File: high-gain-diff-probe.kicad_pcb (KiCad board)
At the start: 2 copper layers, 110 x 80 mm, 94 parts, among them J1 30V DC IN, J2 BNC, J4 BNC, J5 BNC, K1 FTR-B3SA012Z, K2 FTR-B3SA012Z, Q1 2N3906, SW1 MB04L1NCGD, SW2 MB05L1NCGD, SW3 SPDT, SW4 MB04L1NCGD, SW6 SPDT, U1 AD8428BRZ, U2 OP1177AR, U3 BUF634A, U6 LM393, U7 AD8671, U8 BUF634A

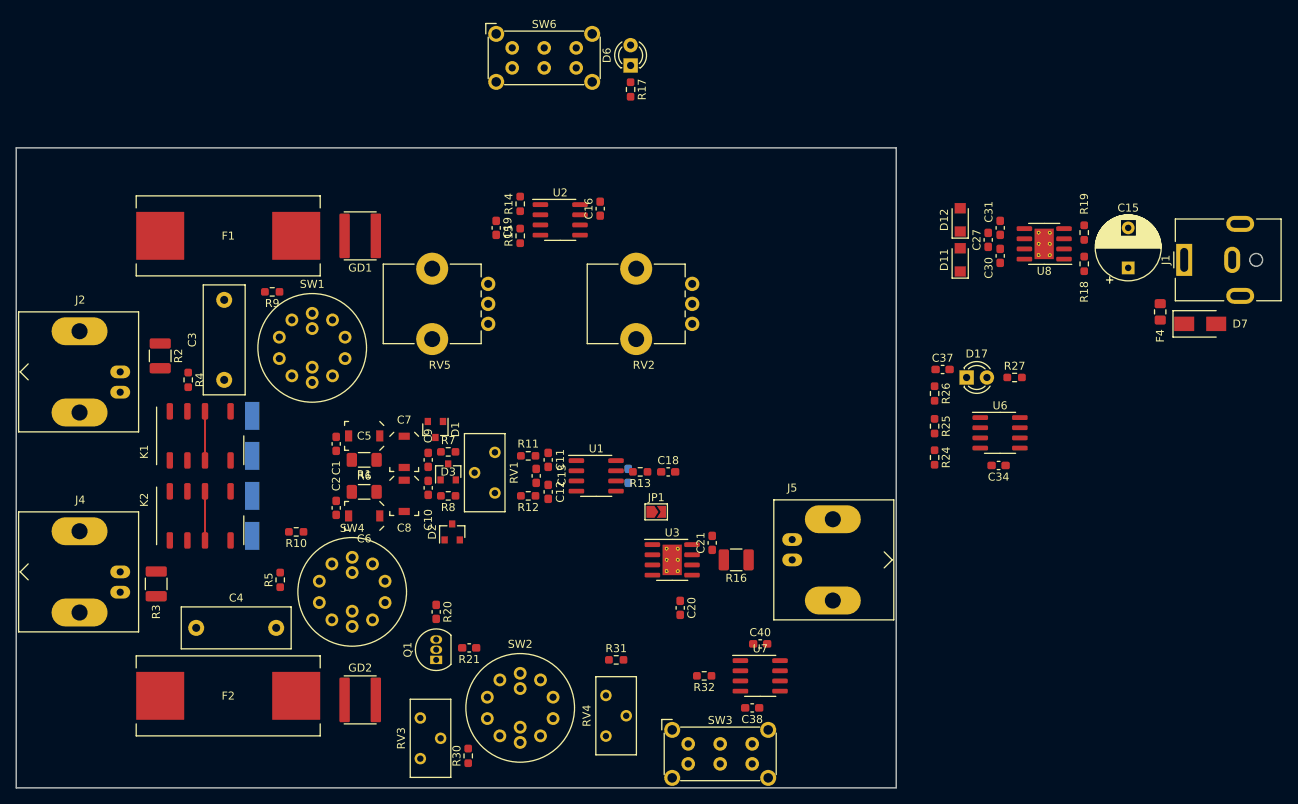
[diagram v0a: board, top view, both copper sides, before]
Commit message: More layout
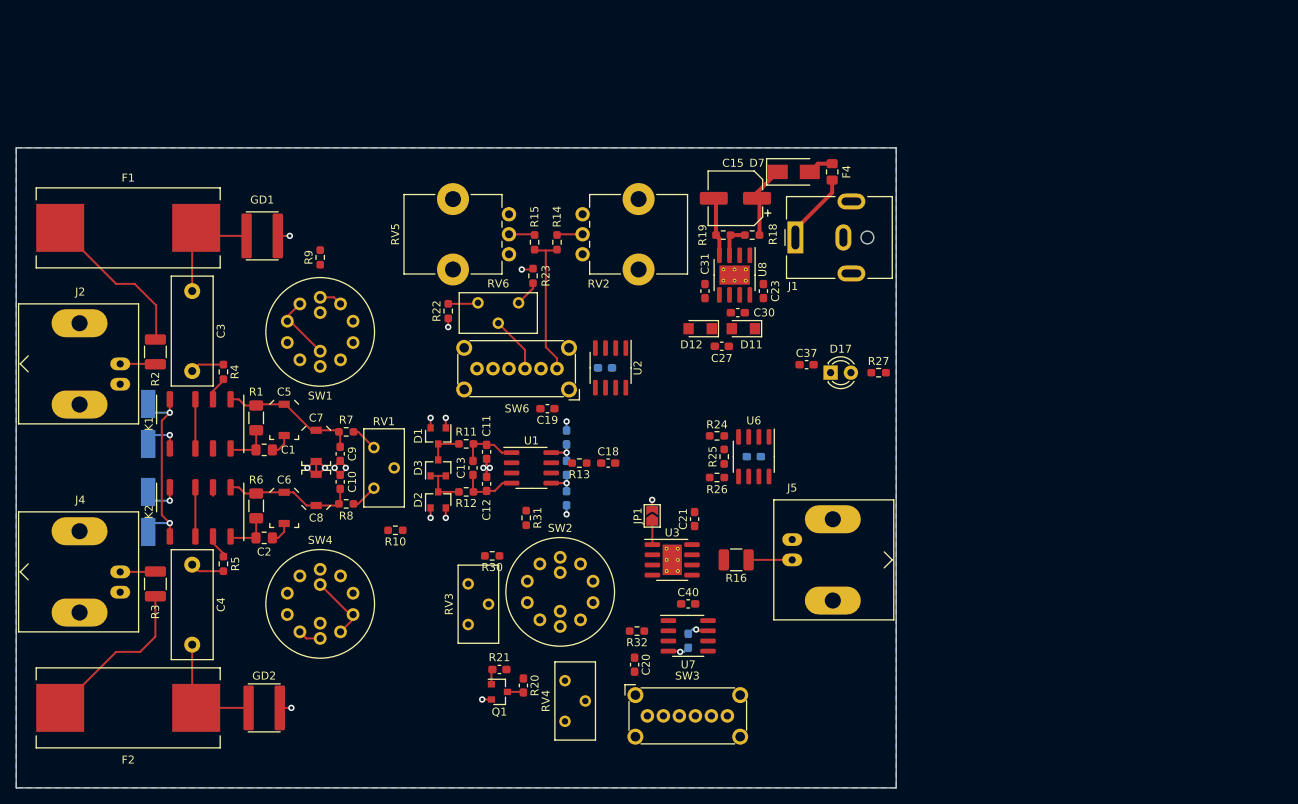
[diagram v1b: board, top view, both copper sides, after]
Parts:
- removed D6: LED, LED_THT:LED_D3.0mm
- removed R17: 15k, Resistor_SMD:R_0603_1608Metric_Pad0.98x0.95mm_HandSolder
- added C17: 1uF, Capacitor_SMD:C_0603_1608Metric_Pad1.05x0.95mm_HandSolder, B.Cu at (158.8, 96.2)
- added C22: 1uF, Capacitor_SMD:C_0603_1608Metric_Pad1.05x0.95mm_HandSolder, B.Cu at (158.8, 103.8)
- added C23: 1uF, Capacitor_SMD:C_0603_1608Metric_Pad1.05x0.95mm_HandSolder, F.Cu at (183.4, 77.9)
- added R22: 10k 0.1%, Resistor_SMD:R_0603_1608Metric_Pad0.98x0.95mm_HandSolder, F.Cu at (144.0, 80.4)
- added R23: 10k 0.1%, Resistor_SMD:R_0603_1608Metric_Pad0.98x0.95mm_HandSolder, F.Cu at (154.6, 76.0)
- added RV6: 200, Potentiometer_THT:Potentiometer_Bourns_3296Y_Vertical, F.Cu at (152.8, 79.4)
- C1, C2: value 20pF -> 22pF; footprint Capacitor_SMD:C_0603_1608Metric_Pad1.05x0.95mm_HandSolder -> Capacitor_SMD:C_0805_2012Metric_Pad1.15x1.40mm_HandSolder
- C15: footprint Capacitor_THT:CP_Radial_D8.0mm_P5.00mm -> Capacitor_SMD:CP_Elec_6.3x7.7
- C16, C34, C38: moved to B.Cu
- Q1: value 2N3906 -> MMBT3906; footprint Package_TO_SOT_THT:TO-92_Inline -> Package_TO_SOT_SMD:SOT-23
- SW3, SW6: footprint Button_Switch_THT:SW_E-Switch_EG2219_DPDT_Angled -> high-gain-diff-probe:SW_TE_1825263-2_DPDT
- moved D7 54.2 mm to (187.2, 63.0)
- moved C15 49.9 mm to (179.9, 66.3), turned to 180 degrees
- moved J1 48.7 mm to (187.4, 71.2)
- moved R19 45.1 mm to (178.4, 70.9), turned to 180 degrees
- moved F4 44.6 mm to (192.0, 63.0)
- moved R18 41.7 mm to (182.0, 70.9), turned to 180 degrees
- moved SW6 40.5 mm to (157.6, 87.6), turned to 180 degrees
- moved U8 38.9 mm to (179.8, 75.9), turned to 270 degrees
- moved C31 37.7 mm to (176.1, 77.9)
- moved C27 35.9 mm to (178.2, 84.8), turned to 180 degrees
- moved D12 35.2 mm to (175.5, 82.6), turned to 180 degrees
- moved C30 33.6 mm to (180.2, 80.6), turned to 180 degrees
- moved U6 30.9 mm to (182.2, 98.6), turned to 270 degrees
- moved C34 30.6 mm to (182.2, 98.6)
- moved R26 29.2 mm to (177.6, 101.2), turned to 0 degrees
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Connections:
- C18 pad 1: SE_SIG -> Net-(C18-Pad1)
- C20 pad 1: SE_SIG -> Net-(C18-Pad1)
- C30 pad 2: Net-(C30-Pad2) -> GND
- C31 pad 1: Net-(C30-Pad2) -> GND
- C8 pad 1: GND -> Net-(C10-Pad2)
- C8 pad 2: Net-(C10-Pad2) -> GND
- D11 pad 2: Net-(C30-Pad2) -> GND
- D12 pad 1: Net-(C30-Pad2) -> GND
- D7 pad 1: Net-(D7-Pad1) -> +15V
- F4 pad 1: +15V -> Net-(D7-Pad2)
- F4 pad 2: Net-(D7-Pad1) -> Net-(F4-Pad2)
- J1 pad 1: Net-(D7-Pad2) -> Net-(F4-Pad2)
- J1 pad MP: (no net) -> Net-(J1-PadMP)
- JP1 pad 1: Net-(JP1-Pad1) -> (no net)
- K1 pad 3: Net-(K1-Pad3) -> ATTEN-
- K1 pad 6: ATTEN- -> Net-(K1-Pad6)
- Q1 pad 1: +15V -> Net-(Q1-Pad1)
- Q1 pad 2: Net-(Q1-Pad2) -> +15V
- R13 pad 1: SE_SIG -> Net-(C18-Pad1)
- R14 pad 1: Net-(C19-Pad2) -> Net-(R14-Pad1)
- R15 pad 2: Net-(C19-Pad2) -> Net-(R14-Pad1)
- R21 pad 2: Net-(Q1-Pad2) -> Net-(Q1-Pad1)
- R4 pad 2: Net-(K1-Pad3) -> Net-(K1-Pad6)
- RV1 pad 1: Net-(R8-Pad1) -> Net-(R7-Pad2)
- RV1 pad 3: Net-(R7-Pad2) -> Net-(R8-Pad1)
- SW1 pad 1: Net-(C3-Pad1) -> Net-(SW1-Pad1)
- SW1 pad 2: GND -> Net-(SW1-Pad1)
- SW1 pad 3: Net-(R9-Pad1) -> Net-(C3-Pad2)
- SW1 pad 4: (no net) -> Net-(C3-Pad2)
- SW1 pad 6: Net-(SW1-Pad6) -> Net-(C3-Pad1)
- SW1 pad 7: Net-(SW1-Pad6) -> GND
- SW1 pad 8: Net-(C3-Pad2) -> Net-(R9-Pad1)
- SW1 pad 9: Net-(C3-Pad2) -> (no net)
- SW1 pad A: Net-(SW1-Pad6) -> Net-(K1-Pad6)
- SW1 pad B: Net-(K1-Pad3) -> Net-(SW1-Pad1)
- SW6 pad 1: GND -> Net-(R14-Pad1)
- SW6 pad 2: Net-(SW6-Pad2) -> Net-(C19-Pad2)
- SW6 pad 3: /REF -> Net-(RV6-Pad2)
- U1 pad 6: Net-(SW6-Pad2) -> /REF
- U3 pad 1: Net-(JP1-Pad1) -> (no net)
- U3 pad 9: (no net) -> -15V
- U6 pad 3: SE_SIG -> /OUT
- U6 pad 6: SE_SIG -> /OUT
- U7 pad 3: SE_SIG -> Net-(C18-Pad1)
- U8 pad 6: Net-(C30-Pad2) -> GND
- U8 pad 9: (no net) -> -15V
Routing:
- net Net-(D18-Pad2): track 0.00 -> 25.5 mm, vias 0 -> 2
- net -15V: track 0.00 -> 24.7 mm, vias 0 -> 7
- net Net-(F2-Pad2): track 0.00 -> 20.6 mm
- net +15V: track 0.00 -> 20.6 mm, vias 0 -> 6
- net Net-(F1-Pad2): track 0.00 -> 20.3 mm
- net GND: track 0.00 -> 19.8 mm, vias 0 -> 10
- net Net-(R14-Pad1): track 0.00 -> 18.2 mm
- net Net-(C4-Pad2): track 0.00 -> 17.5 mm
- net Net-(C5-Pad1): track 0.00 -> 17.3 mm
- net Net-(C3-Pad2): track 0.00 -> 17.0 mm
- net Net-(C10-Pad2): track 0.00 -> 16.6 mm
- net Net-(F4-Pad2): track 0.00 -> 9.08 mm
- net Net-(SW4-Pad6): track 0.00 -> 8.47 mm
- net Net-(SW1-Pad1): track 0.00 -> 8.47 mm
- net ATTEN+: track 0.00 -> 7.56 mm
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- added copper zone on In2.Cu, net +15V
- added copper zone on B.Cu, net -15V
- added copper zone on In1.Cu, net GND
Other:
- copper layers 2 -> 4
